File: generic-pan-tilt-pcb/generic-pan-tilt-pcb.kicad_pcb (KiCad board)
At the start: 2 copper layers, 85 x 50 mm, 86 parts, among them J1 B4P-VH-FB-B, J10 USB4115-03-C, J11 Conn_01x08, J12 Conn_01x08, J13 Conn_01x05, J2 NC5MAV, J3 NC5FAV, J5 BM03B-SRSS-TB, J7 BM03B-SRSS-TB, J8 B12B-PH-SM4-TB, J9 B12B-PH-SM4-TB, SW1 PTS 647 SK70 SMTR2 LFS, SW2 PTS 647 SK70 SMTR2 LFS, SW3 219-12LPST, U1 RP2040, U2 W25Q128JVS, U3 AP63203WU, U4 ISO1450DW, U5 MCP23017_SO, U6 LIS3DH, Y1 ABM8-272-T3

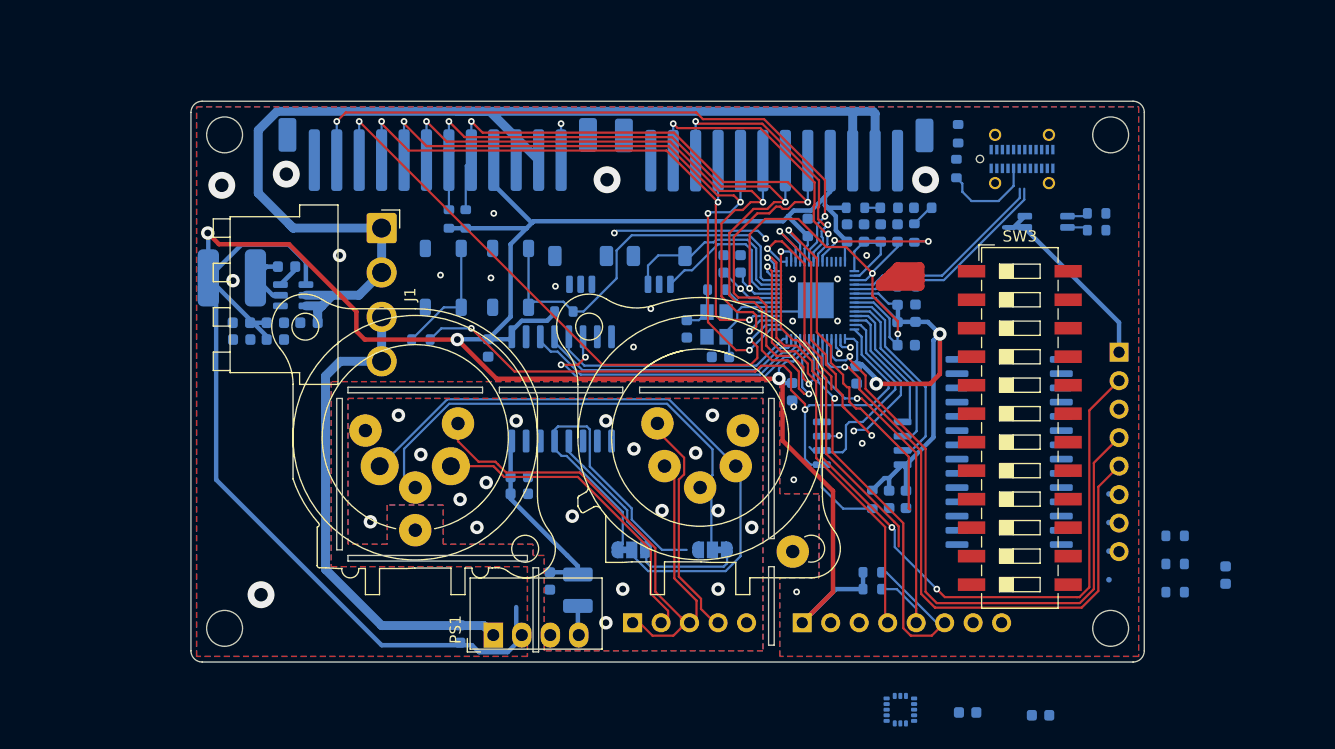
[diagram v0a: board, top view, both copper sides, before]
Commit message: make board bigger
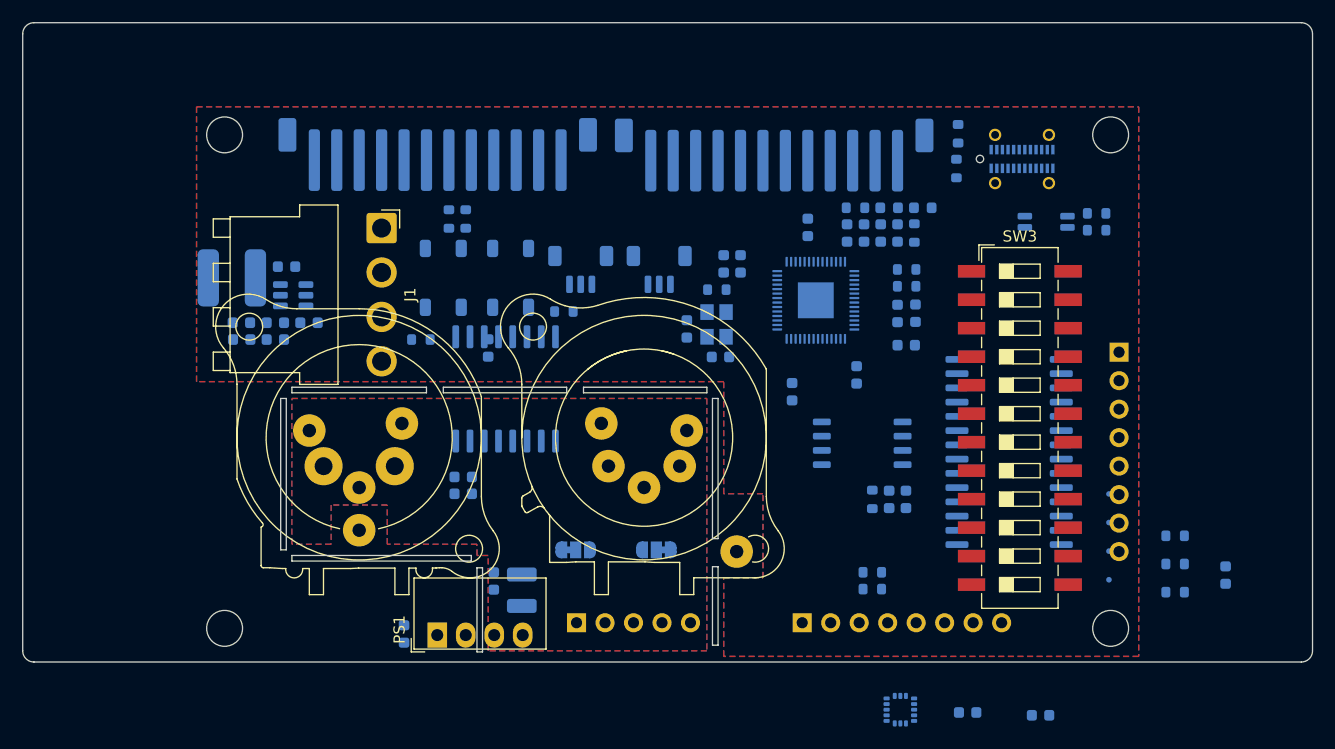
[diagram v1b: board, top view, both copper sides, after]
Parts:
- moved C23 5.00 mm to (115.0, 121.0)
- moved C25 5.00 mm to (120.3, 107.0)
- moved C26 5.00 mm to (123.0, 116.3)
- moved C27 5.00 mm to (120.3, 108.5)
- moved J13 5.00 mm to (130.4, 120.0)
- moved J2 5.00 mm to (111.0, 103.5)
- moved J3 5.00 mm to (136.4, 103.5)
- moved JP1 5.00 mm to (137.5, 113.5)
- moved JP2 5.00 mm to (130.3, 113.5)
- moved L2 5.00 mm to (125.5, 117.1)
- moved PS1 5.00 mm to (118.0, 121.1)
- moved U4 5.00 mm to (124.1, 99.2)
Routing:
- net +3V3: track 342.8 -> 0.00 mm, vias 6 -> 0
- net +24V: track 107.8 -> 0.00 mm
- net /I2C_MOT_SCL: track 75.4 -> 0.00 mm, vias 3 -> 0
- net /I2C_MOT_SDA: track 74.7 -> 0.00 mm, vias 3 -> 0
- net /EXP_CS0: track 72.0 -> 0.00 mm, vias 3 -> 0
- net GND: track 66.9 -> 0.00 mm, vias 25 -> 0
- net /BOOTSEL: track 66.8 -> 0.00 mm, vias 2 -> 0
- net /SPI_MOT_POCI: track 61.0 -> 0.00 mm, vias 4 -> 0
- net /SPI_MOT_SCK: track 59.6 -> 0.00 mm, vias 3 -> 0
- net /SPI_MOT_CS_MOT0_GPIO: track 57.7 -> 0.00 mm, vias 2 -> 0
- net /EXP_IRQ0: track 57.6 -> 0.00 mm, vias 1 -> 0
- net /RS485_B-: track 57.5 -> 0.00 mm
- net /SPI_MOT_PICO: track 56.4 -> 0.00 mm, vias 3 -> 0
- net /EXP_IRQ1: track 56.0 -> 0.00 mm, vias 1 -> 0
- net /SPI_MOT_CS_MOT0_CNTLR: track 53.2 -> 0.00 mm, vias 2 -> 0
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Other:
- board size 85 x 50 mm -> 115 x 57 mm
